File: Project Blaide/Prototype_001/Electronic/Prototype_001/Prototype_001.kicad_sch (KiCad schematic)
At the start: 0 parts

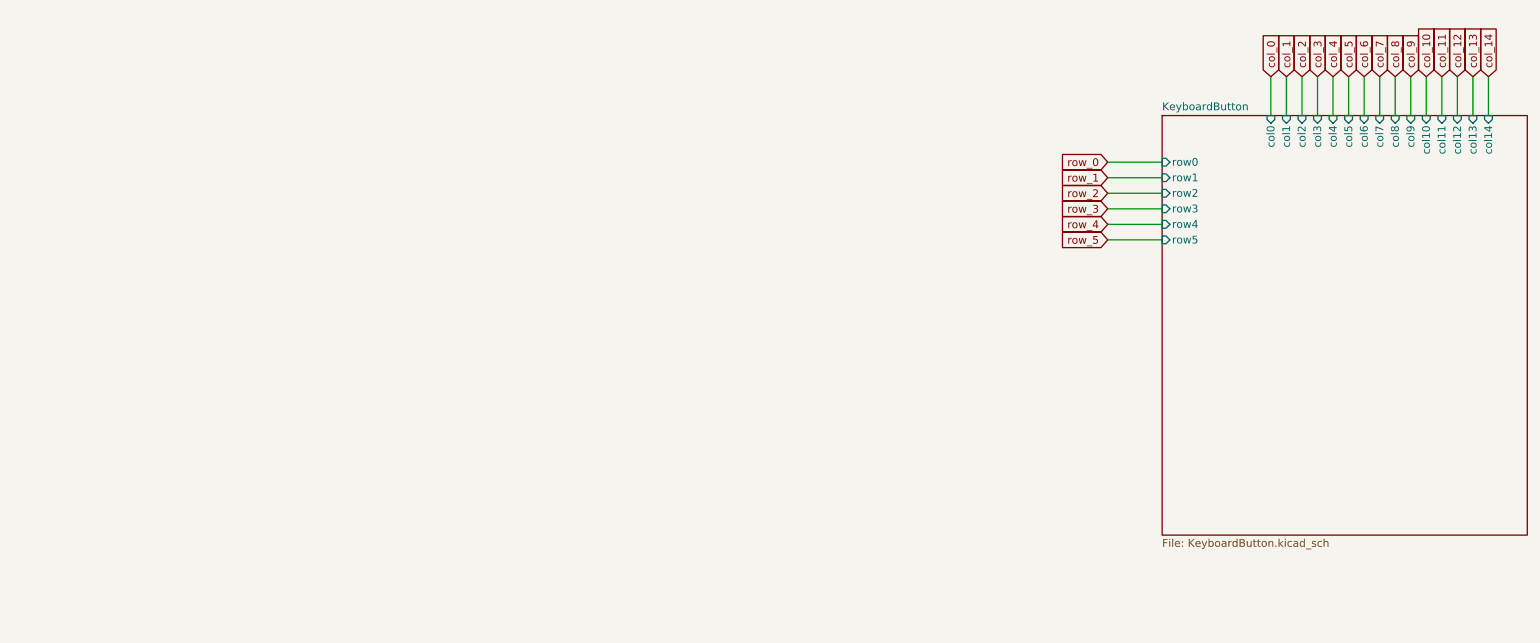
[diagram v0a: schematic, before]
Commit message: Ivan - Update: v0.0.0.1 - Finalizing electronic Board
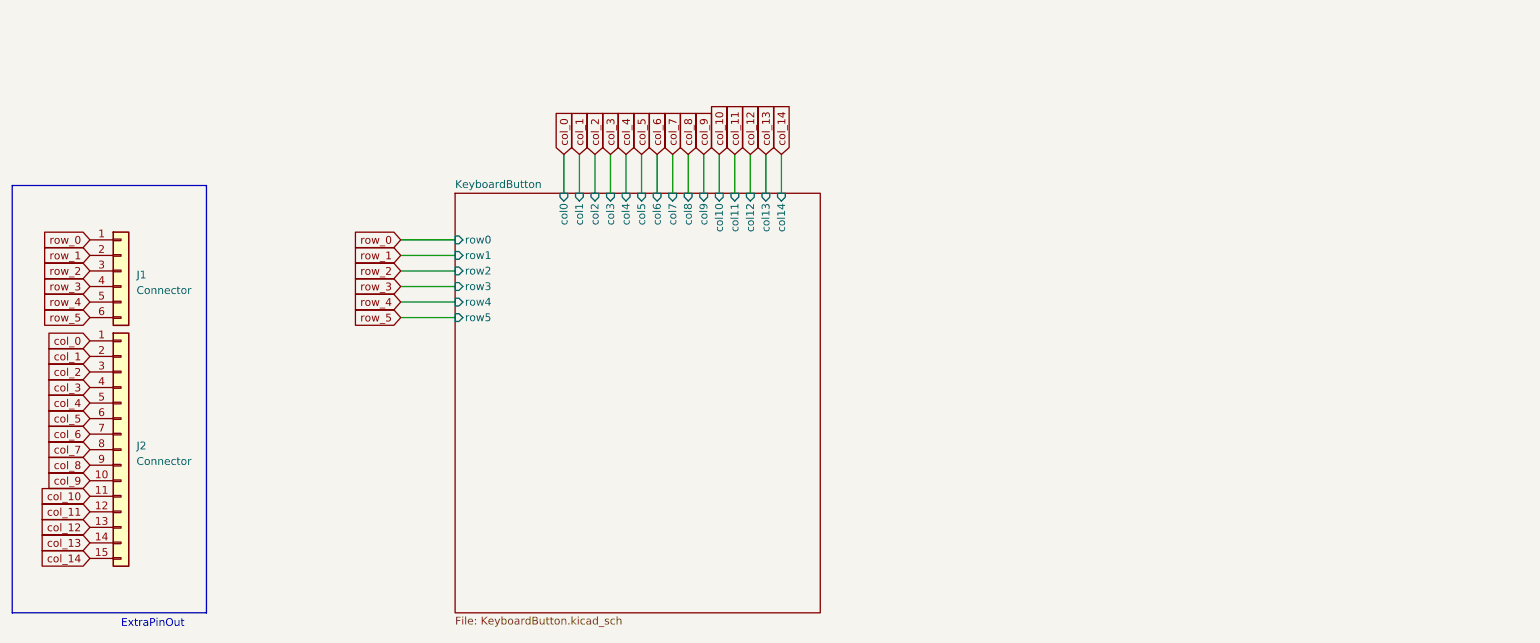
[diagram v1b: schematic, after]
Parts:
- added J1: Connector, Connector_PinHeader_2.54mm:PinHeader_1x06_P2.54mm_Vertical, symbol Connector_Generic:Conn_01x06
- added J2: Connector, Connector_PinHeader_2.54mm:PinHeader_1x15_P2.54mm_Vertical, symbol Connector_Generic:Conn_01x15
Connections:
- net col_0: now also J2.1 (Pin_1)
- net col_1: now also J2.2 (Pin_2)
- net col_10: now also J2.11 (Pin_11)
- net col_11: now also J2.12 (Pin_12)
- net col_12: now also J2.13 (Pin_13)
- net col_13: now also J2.14 (Pin_14)
- net col_14: now also J2.15 (Pin_15)
- net col_2: now also J2.3 (Pin_3)
- net col_3: now also J2.4 (Pin_4)
- net col_4: now also J2.5 (Pin_5)
- net col_5: now also J2.6 (Pin_6)
- net col_6: now also J2.7 (Pin_7)
- net col_7: now also J2.8 (Pin_8)
- net col_8: now also J2.9 (Pin_9)
- net col_9: now also J2.10 (Pin_10)
- net row_0: now also J1.1 (Pin_1)
- net row_1: now also J1.2 (Pin_2)
- net row_2: now also J1.3 (Pin_3)
- net row_3: now also J1.4 (Pin_4)
- net row_4: now also J1.5 (Pin_5)
- net row_5: now also J1.6 (Pin_6)
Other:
- note added: "ExtraPinOut"
